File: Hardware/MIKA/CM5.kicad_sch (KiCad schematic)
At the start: 16 parts, among them J3 PWR_BUTT, J4 Fan Header, J5 RPI Pin-Header, SW1 SW_Push, SW2 SW_Push

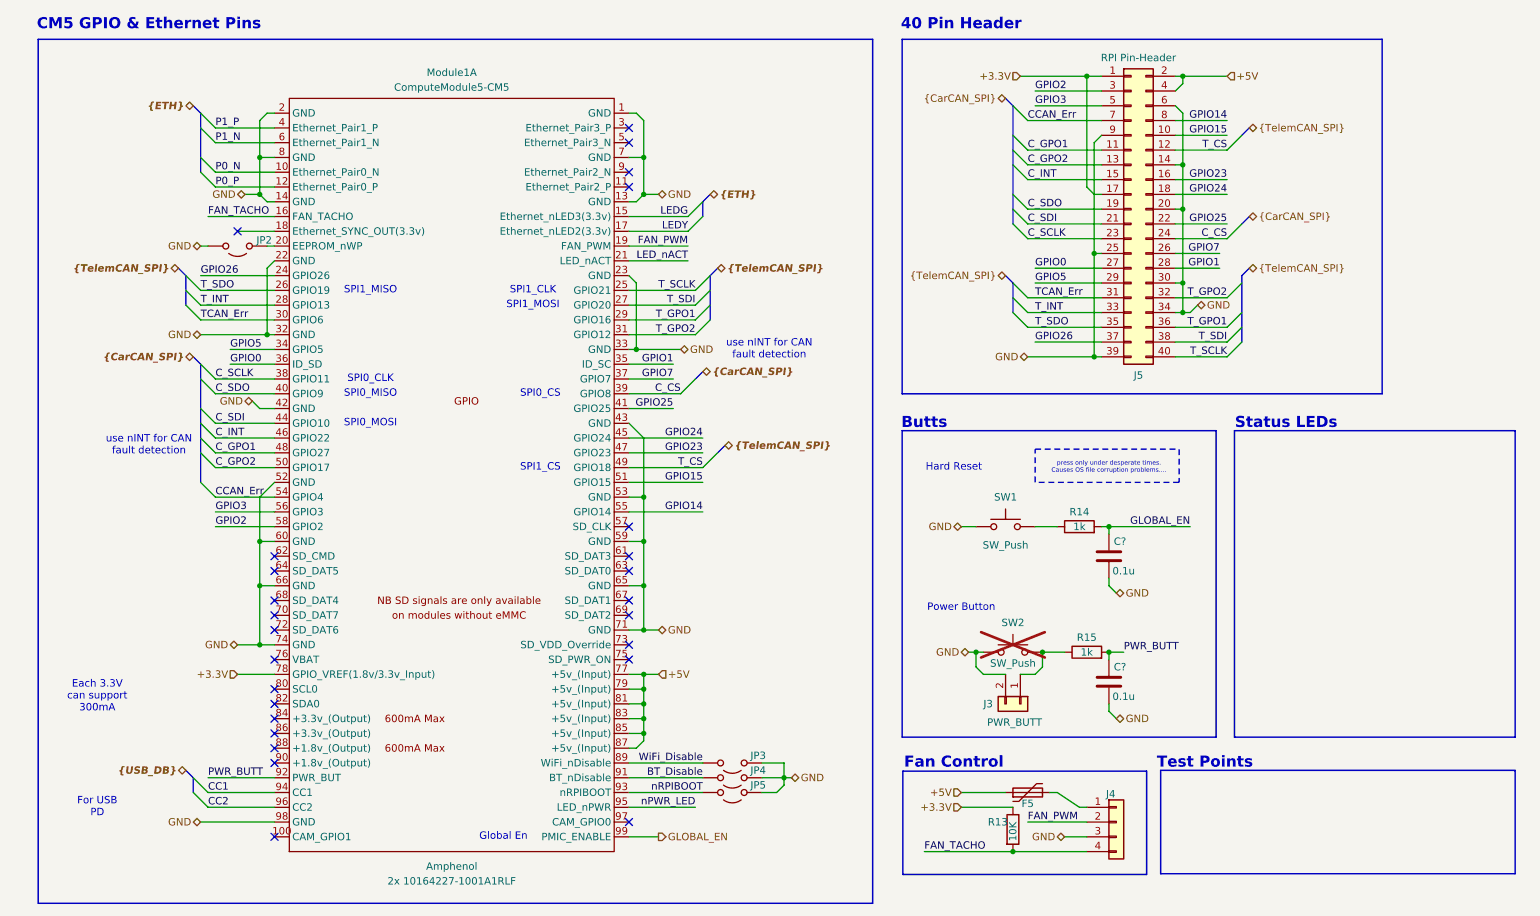
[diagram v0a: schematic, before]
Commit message: bahasdf;ladjsfhadf boooooooooooshksa
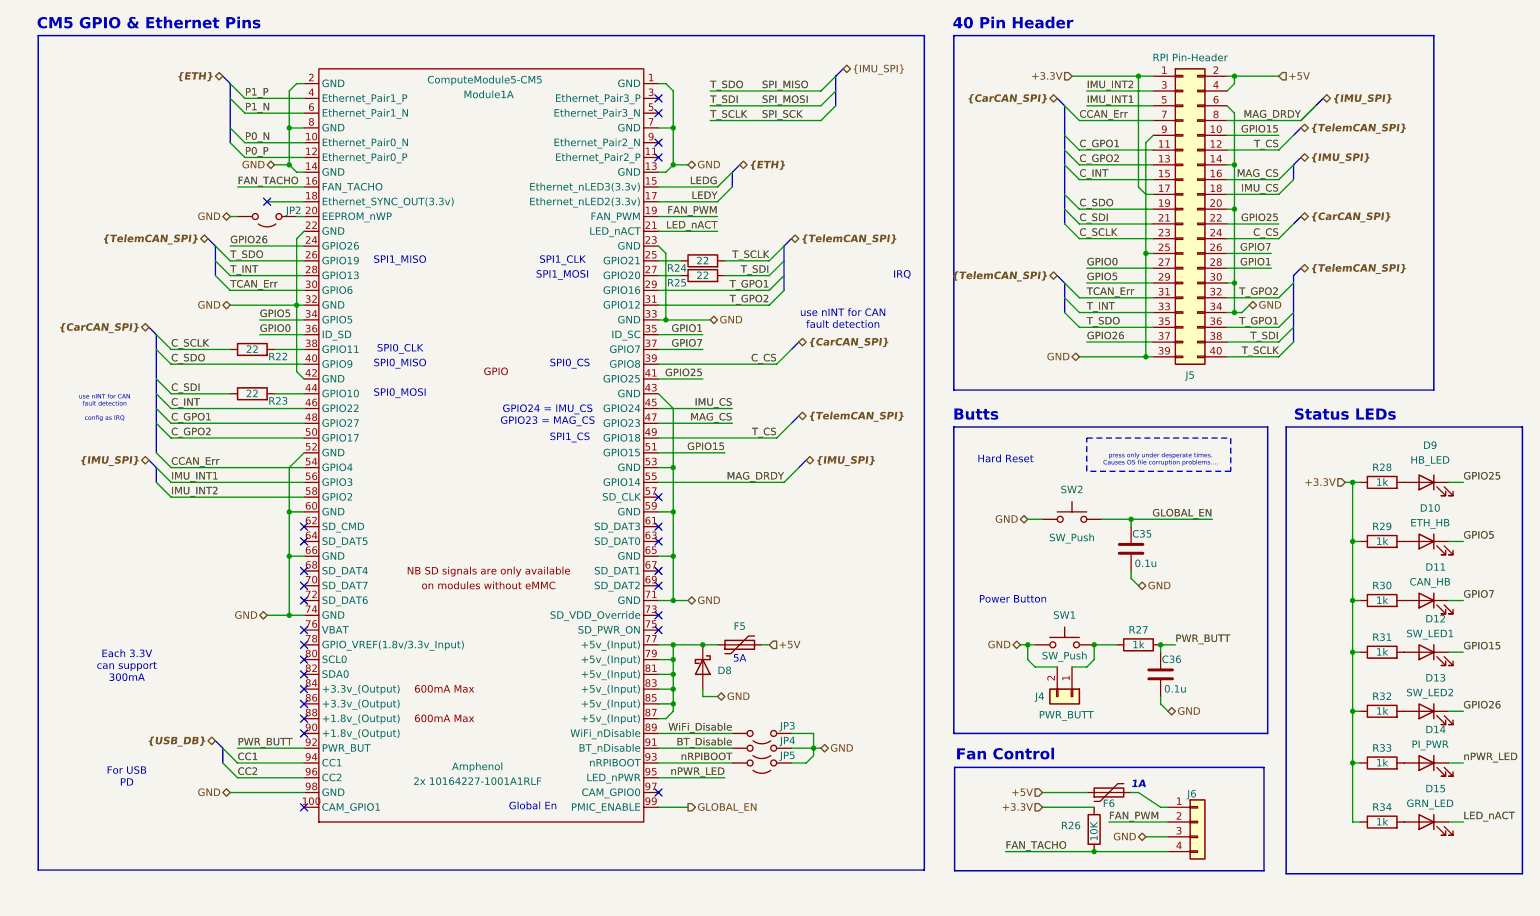
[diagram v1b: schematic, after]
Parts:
- removed R14: 1k, symbol Device:R
- added D10: ETH_HB, symbol Device:LED
- added D11: CAN_HB, symbol Device:LED
- added D12: SW_LED1, symbol Device:LED
- added D13: SW_LED2, symbol Device:LED
- added D14: PI_PWR, symbol Device:LED
- added D15: GRN_LED, symbol Device:LED
- added D8: D_Schottky, symbol Device:D_Schottky
- added D9: HB_LED, symbol Device:LED
- added F5: Polyfuse, symbol Device:Polyfuse
- added R22, R23, R24, R25: 22, symbol Device:R
- added R28, R29, R30, R31, R32, R33, R34: 1k, symbol Device:R
- SW1: renamed from SW2; now fitted
- gave numbers to parts that had none: 2
- renumbered F5 to F6, J3 to J4, J4 to J6, R13 to R26, R15 to R27, SW1 to SW2
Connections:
- net +3.3V: now also R28.1, R29.1, R30.1, R31.1, R32.1, R33.1, R34.1; no longer Module1.78 (GPIO_VREF(1.8v/3.3v_Input))
- net +5V: now also F5.2; no longer Module1.77 (+5v_(Input)), Module1.79 (+5v_(Input)), Module1.81 (+5v_(Input)), Module1.83 (+5v_(Input)), Module1.85 (+5v_(Input)), Module1.87 (+5v_(Input))
- net C_SCLK: now also R22.1; no longer Module1.38 (GPIO11)
- net C_SDI: now also R23.1; no longer Module1.44 (GPIO10)
- net GLOBAL_EN: now also SW2.2
- net GND: now also D8.2 (A)
- net GPIO15: now also D12.1 (K)
- net GPIO25: now also D9.1 (K)
- net GPIO26: now also D13.1 (K)
- net GPIO5: now also D10.1 (K)
- net GPIO7: now also D11.1 (K)
- net LED_nACT: now also D15.1 (K)
- net nPWR_LED: now also D14.1 (K)
- net GPIO14 renamed MAG_DRDY
- net GPIO2 renamed IMU_INT2
- net GPIO23 renamed MAG_CS
- net GPIO24 renamed IMU_CS
- net GPIO3 renamed IMU_INT1
- net T_SCLK: no longer names the net of Module1.25 (GPIO21)
- net T_SCLK: now also R24.1; no longer J5.40 (Pin_40)
- net T_SDI: no longer names the net of Module1.27 (GPIO20)
- net T_SDI: now also R25.1; no longer J5.38 (Pin_38)
- net T_SDO renamed SPI_MISO
- new net: Module1.38 (GPIO11), R22.2
- new net: Module1.44 (GPIO10), R23.2
- new net: D8.1 (K), F5.1, Module1.77 (+5v_(Input)), Module1.79 (+5v_(Input)), Module1.81 (+5v_(Input)), Module1.83 (+5v_(Input)), Module1.85 (+5v_(Input)), Module1.87 (+5v_(Input))
- new net: D14.2 (A), R33.2
- new net: D9.2 (A), R28.2
- new net: D11.2 (A), R30.2
- new net: D15.2 (A), R34.2
- new net: D13.2 (A), R32.2
- new net: D12.2 (A), R31.2
- new net: D10.2 (A), R29.2
- new net SPI_MOSI: J5.38 (Pin_38), R25.2
- new net SPI_SCK: J5.40 (Pin_40), R24.2
- no-connect marks 26 -> 27
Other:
- note added: "1A"
- note added: "5A"
- note added: "GPIO24 = IMU_CS GPIO23 = MAG_CS"
- note added: "IRQ"
- note added: "use nINT for CAN fault detection config as IRQ"
- note removed: "Test Points"
- moved on the sheet: C35, C36, F6, J4, J5, J6, JP2, JP3, JP4, JP5, Module1A, R26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
